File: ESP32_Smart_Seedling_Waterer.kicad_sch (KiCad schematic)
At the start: 23 parts, among them J1 Solenoid_12V, J2 AM2302 ~ DHT22, J3 Barrel_Jack_Switch, K1 SRD-05VDC-SL-C, Q1 PN2222A, Q2 PN2222A, SW1 SW_Push, SW3 SW_SPST, U1 LM7805_TO220, U2 ESP32-C3 SuperMini

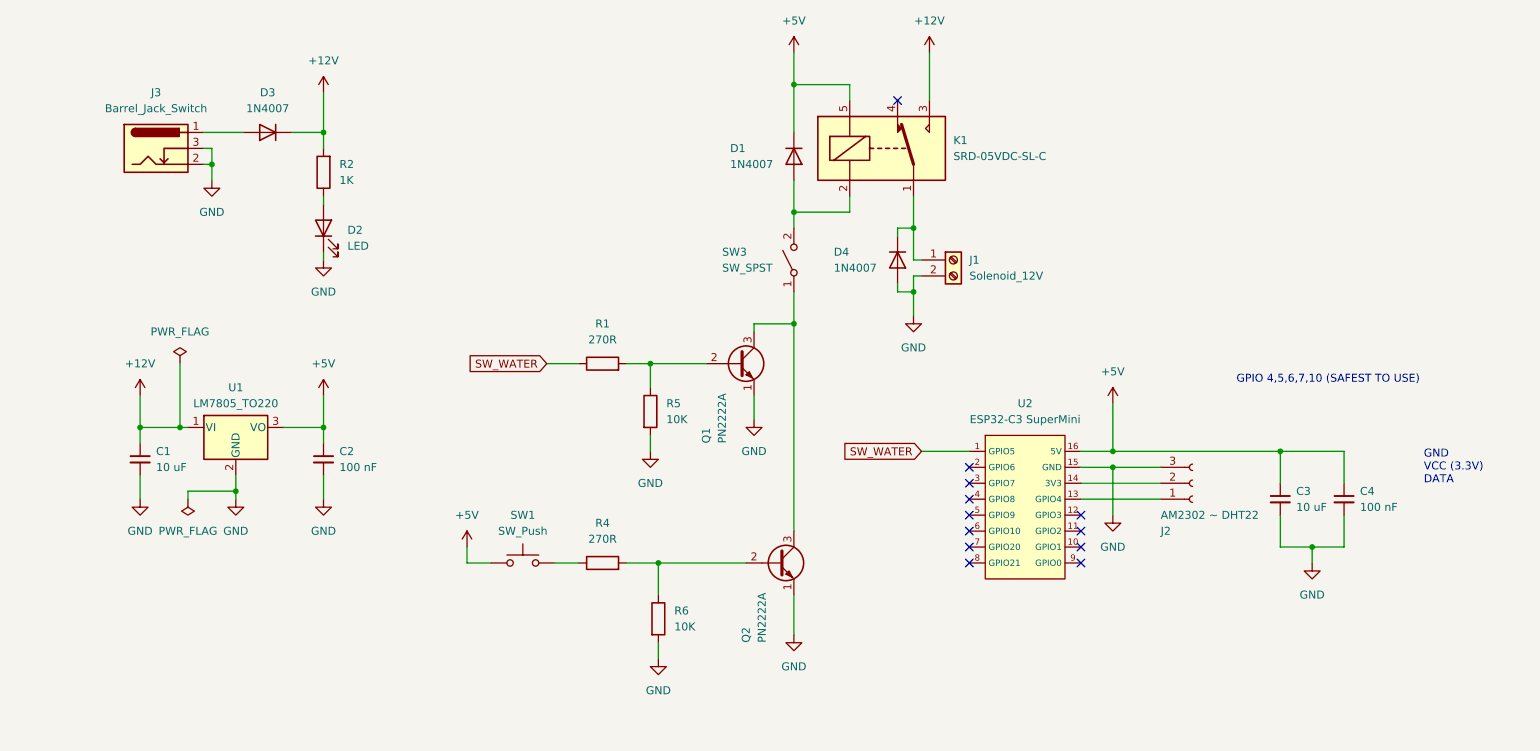
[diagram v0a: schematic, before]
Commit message: 9.5.2026 rtc added
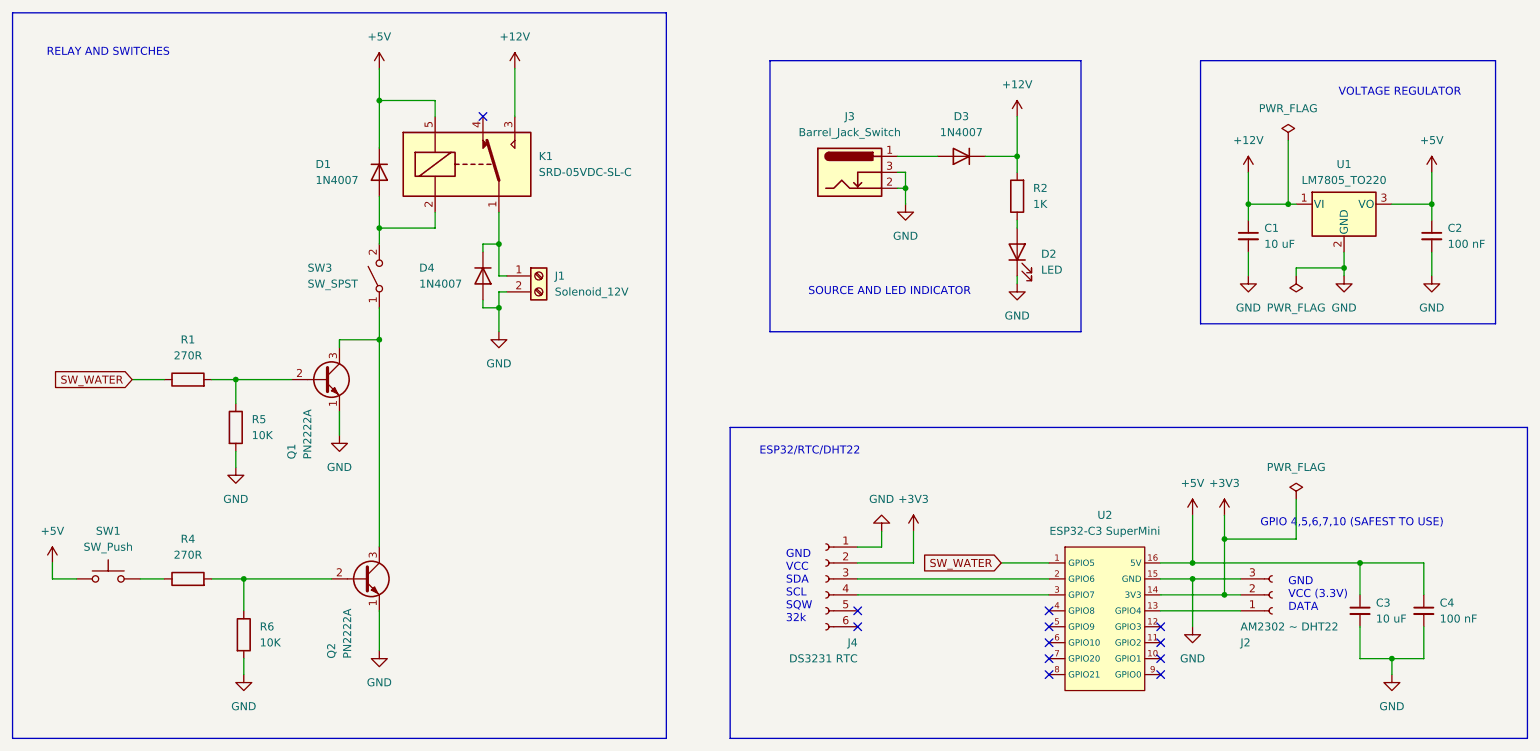
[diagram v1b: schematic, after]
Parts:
- added J4: DS3231 RTC, Connector_PinSocket_2.54mm:PinSocket_1x06_P2.54mm_Vertical, symbol Connector:Conn_01x06_Socket
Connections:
- net GND: now also J4.1 (Pin_1)
- net +3V3: now reaches J2.2 (Pin_2), U2.14 (3V3)
- net +3V3: now also J4.2 (Pin_2)
- net at U2.2 (GPIO6): now also J4.3 (Pin_3)
- net at U2.3 (GPIO7): now also J4.4 (Pin_4)
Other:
- note added: "ESP32/RTC/DHT22"
- note added: "GND VCC SDA SCL SQW 32k"
- note added: "RELAY AND SWITCHES"
- note added: "SOURCE AND LED INDICATOR"
- note added: "VOLTAGE REGULATOR"
- moved on the sheet: C1, C2, C3, C4, D1, D2, D3, D4, J1, J2, J3, K1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
